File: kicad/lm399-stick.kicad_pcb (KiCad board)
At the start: 4 copper layers, 48.3 x 16.5 mm, 18 parts, among them P1 CONN_1X1, P2 CONN_1X1, P3 CONN_1X1, P4 CONN_1X1, P5 CONN_2X1, U1 LM399A, U2 OP07

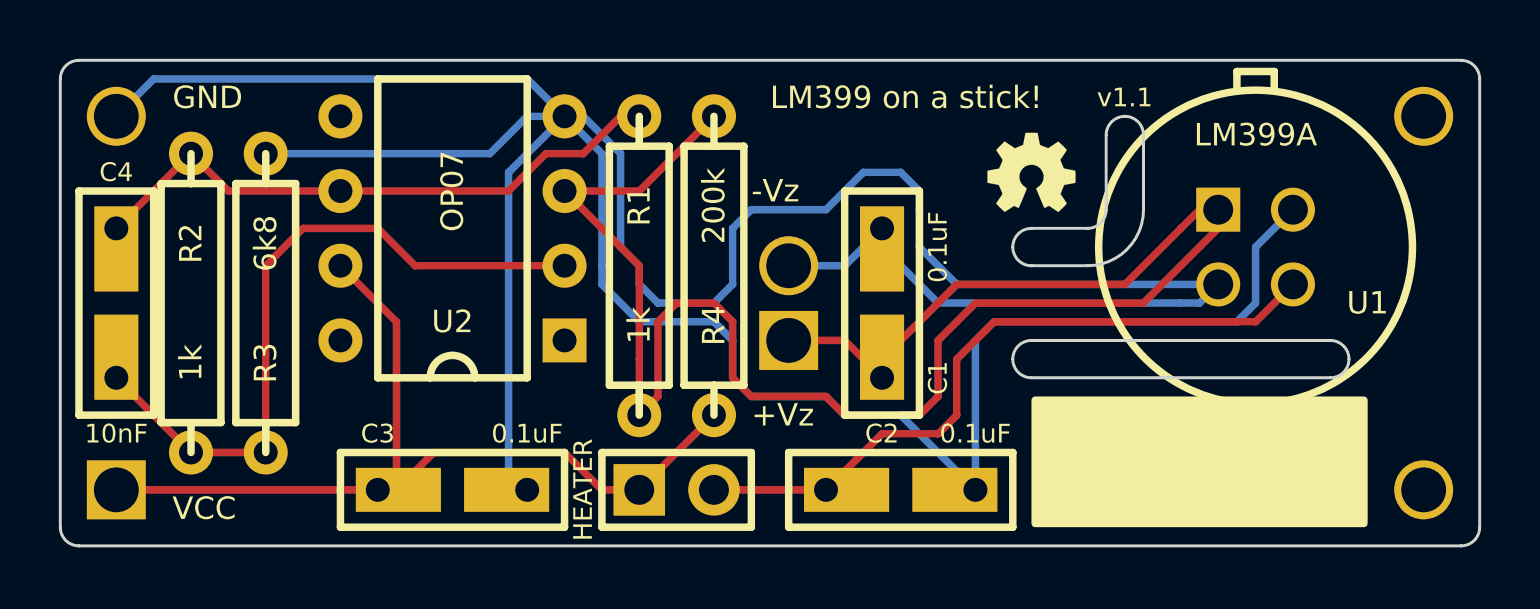
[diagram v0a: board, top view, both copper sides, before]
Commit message: v1.1
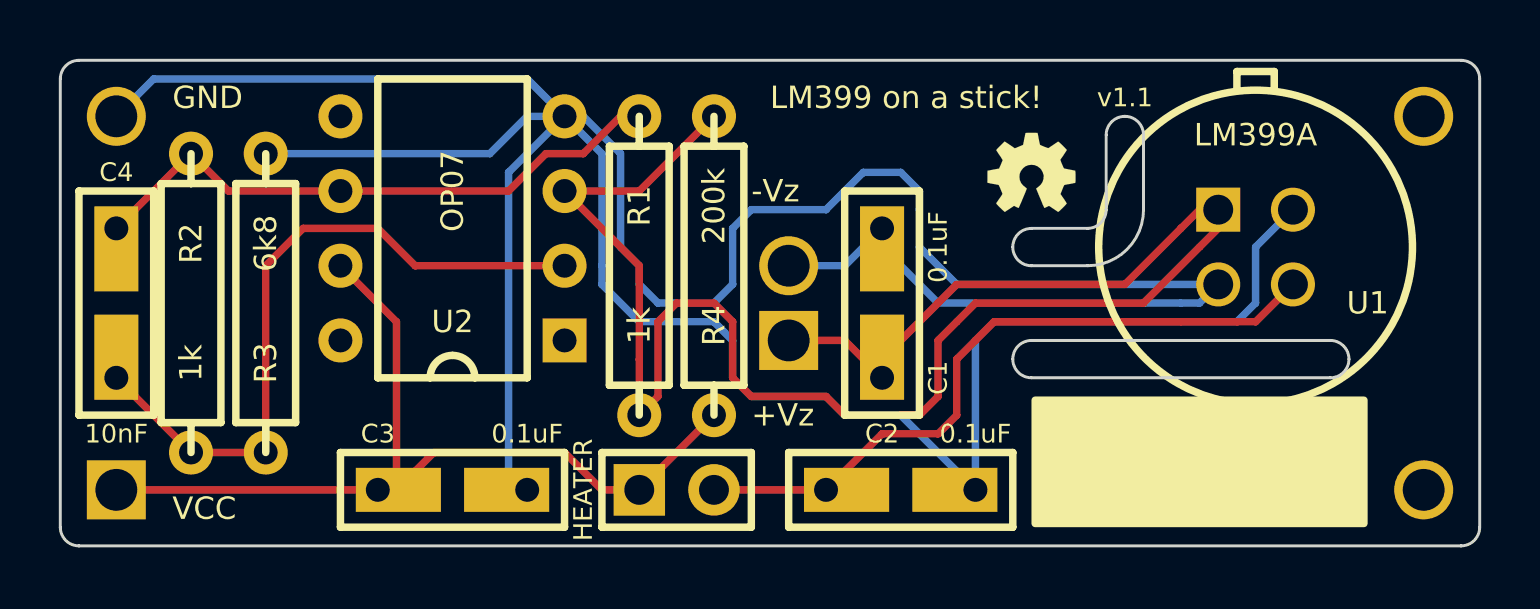
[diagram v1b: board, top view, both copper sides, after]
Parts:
- removed the H*** at (209.6, 137.2)
- removed the H*** at (209.6, 149.9)
- added H***: Val**, 1pin_056_079, F.Cu at (209.6, 137.2)
- added H***: Val**, 1pin_056_079, F.Cu at (209.6, 149.9)
- P1, P2, P3, P4: footprint 1pin_060_079 -> 1pin_056_079
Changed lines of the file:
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@@
     (links 25)
     (no_connects 0)
-    (area 160.203445 133.731 212.753222 153.289)
+    (area 163.144999 135.204999 211.505001 151.815001)
     (thickness 1.6)
     (drawings 32)
@@
     (mod_text_width 0.15)
     (pad_size 2.0066 2.0066)
-    (pad_drill 1.524)
+    (pad_drill 1.4224)
     (pad_to_mask_clearance 0)
     (aux_axis_origin 0 0)
@@
       (xy -0.90932 1.3462)) (layer F.SilkS) (width 0.00254))
   )
-  (module 1pin_060_079 (layer F.Cu)
+  (module 1pin_056_079 (layer F.Cu)
+    (at 165.1 137.16)
+    (descr "1 pin, 0.056\" drill, 0.079\" round pad")
+    (fp_text reference P2 (at 0 -2.54) (layer F.SilkS) hide
+      (effects (font (size 1.016 1.016) (thickness 0.254)))
+    )
+    (fp_text value CONN_1X1 (at 0 2.54) (layer F.SilkS) hide
+      (effects (font (size 1.016 1.016) (thickness 0.254)))
+    )
+    (pad 1 thru_hole circle (at 0 0) (size 2.0066 2.0066) (drill 1.4224)
+      (layers *.Cu *.Mask F.SilkS)
+      (net 2 -Vz)
+    )
+  )
+  (module 1pin_056_079 (layer F.Cu)
     (at 209.55 137.16)
-    (descr "1 pin, 0.060\" drill, 0.079\" round pad")
+    (descr "1 pin, 0.056\" drill, 0.079\" round pad")
     (path 1pin)
     (fp_text reference H*** (at 0 -2.54) (layer F.SilkS) hide
@@
       (effects (font (size 1.016 1.016) (thickness 0.254)))
     )
-    (pad 1 thru_hole circle (at 0 0) (size 2.0066 2.0066) (drill 1.524)
-      (layers *.Cu *.Mask F.SilkS)
-    )
-  )
-  (module 1pin_060_079 (layer F.Cu)
+    (pad 1 thru_hole circle (at 0 0) (size 2.0066 2.0066) (drill 1.4224)
+      (layers *.Cu *.Mask F.SilkS)
+    )
+  )
+  (module 1pin_056_079 (layer F.Cu)
     (at 209.55 149.86)
-    (descr "1 pin, 0.060\" drill, 0.079\" round pad")
+    (descr "1 pin, 0.056\" drill, 0.079\" round pad")
     (path 1pin)
     (fp_text reference H*** (at 0 -2.54) (layer F.SilkS) hide
@@
       (effects (font (size 1.016 1.016) (thickness 0.254)))
     )
-    (pad 1 thru_hole circle (at 0 0) (size 2.0066 2.0066) (drill 1.524)
-      (layers *.Cu *.Mask F.SilkS)
-    )
-  )
-  (module 1pin_060_079 (layer F.Cu)
+    (pad 1 thru_hole circle (at 0 0) (size 2.0066 2.0066) (drill 1.4224)
+      (layers *.Cu *.Mask F.SilkS)
+    )
+  )
+  (module 1pin_056_079 (layer F.Cu)
     (at 165.1 149.86)
-    (descr "1 pin, 0.060\" drill, 0.079\" round pad")
+    (descr "1 pin, 0.056\" drill, 0.079\" round pad")
     (fp_text reference P1 (at 0 -2.54) (layer F.SilkS) hide
       (effects (font (size 1.016 1.016) (thickness 0.254)))
@@
       (effects (font (size 1.016 1.016) (thickness 0.254)))
     )
-    (pad 1 thru_hole rect (at 0 0) (size 2.0066 2.0066) (drill 1.524)
+    (pad 1 thru_hole rect (at 0 0) (size 2.0066 2.0066) (drill 1.4224)
       (layers *.Cu *.Mask F.SilkS)
       (net 6 Vcc)
     )
   )
-  (module 1pin_060_079 (layer F.Cu)
-    (at 165.1 137.16)
-    (descr "1 pin, 0.060\" drill, 0.079\" round pad")
-    (fp_text reference P2 (at 0 -2.54) (layer F.SilkS) hide
+  (module 1pin_056_079 (layer F.Cu)
+    (at 187.96 142.24)
+    (descr "1 pin, 0.056\" drill, 0.079\" round pad")
+    (fp_text reference P4 (at 0 -2.54) (layer F.SilkS) hide
       (effects (font (size 1.016 1.016) (thickness 0.254)))
     )
@@
       (effects (font (size 1.016 1.016) (thickness 0.254)))
     )
-    (pad 1 thru_hole circle (at 0 0) (size 2.0066 2.0066) (drill 1.524)
-      (layers *.Cu *.Mask F.SilkS)
-      (net 2 -Vz)
-    )
-  )
-  (module 1pin_060_079 (layer F.Cu)
-    (at 187.96 142.24)
-    (descr "1 pin, 0.060\" drill, 0.079\" round pad")
-    (fp_text reference P4 (at 0 -2.54) (layer F.SilkS) hide
+    (pad 1 thru_hole circle (at 0 0) (size 2.0066 2.0066) (drill 1.4224)
+      (layers *.Cu *.Mask F.SilkS)
+      (net 2 -Vz)
+    )
+  )
+  (module 1pin_056_079 (layer F.Cu)
+    (at 187.96 144.78)
+    (descr "1 pin, 0.056\" drill, 0.079\" round pad")
+    (fp_text reference P3 (at 0 -2.54) (layer F.SilkS) hide
       (effects (font (size 1.016 1.016) (thickness 0.254)))
     )
@@
       (effects (font (size 1.016 1.016) (thickness 0.254)))
     )
-    (pad 1 thru_hole circle (at 0 0) (size 2.0066 2.0066) (drill 1.524)
-      (layers *.Cu *.Mask F.SilkS)
-      (net 2 -Vz)
-    )
-  )
-  (module 1pin_060_079 (layer F.Cu)
-    (at 187.96 144.78)
-    (descr "1 pin, 0.060\" drill, 0.079\" round pad")
-    (fp_text reference P3 (at 0 -2.54) (layer F.SilkS) hide
-      (effects (font (size 1.016 1.016) (thickness 0.254)))
-    )
-    (fp_text value CONN_1X1 (at 0 2.54) (layer F.SilkS) hide
-      (effects (font (size 1.016 1.016) (thickness 0.254)))
-    )
-    (pad 1 thru_hole rect (at 0 0) (size 2.0066 2.0066) (drill 1.524)
+    (pad 1 thru_hole rect (at 0 0) (size 2.0066 2.0066) (drill 1.4224)
       (layers *.Cu *.Mask F.SilkS)
       (net 1 +Vz)
